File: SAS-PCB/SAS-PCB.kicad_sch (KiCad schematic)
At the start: 23 parts, among them J1_Batt1 691137710002, J2-LCD1 Conn_01x04_Socket, J3-LCD2 Conn_01x04_Socket, J4-BMP280 Conn_01x06_Pin, J5-GPS1 Conn_01x04_Socket, J6-cable-plat1 Conn_02x20_Odd_Even, J7-RFD900x1 691137710002, J8-Fan1 Conn_01x04_Socket, J9-Fan2 Conn_01x04_Socket

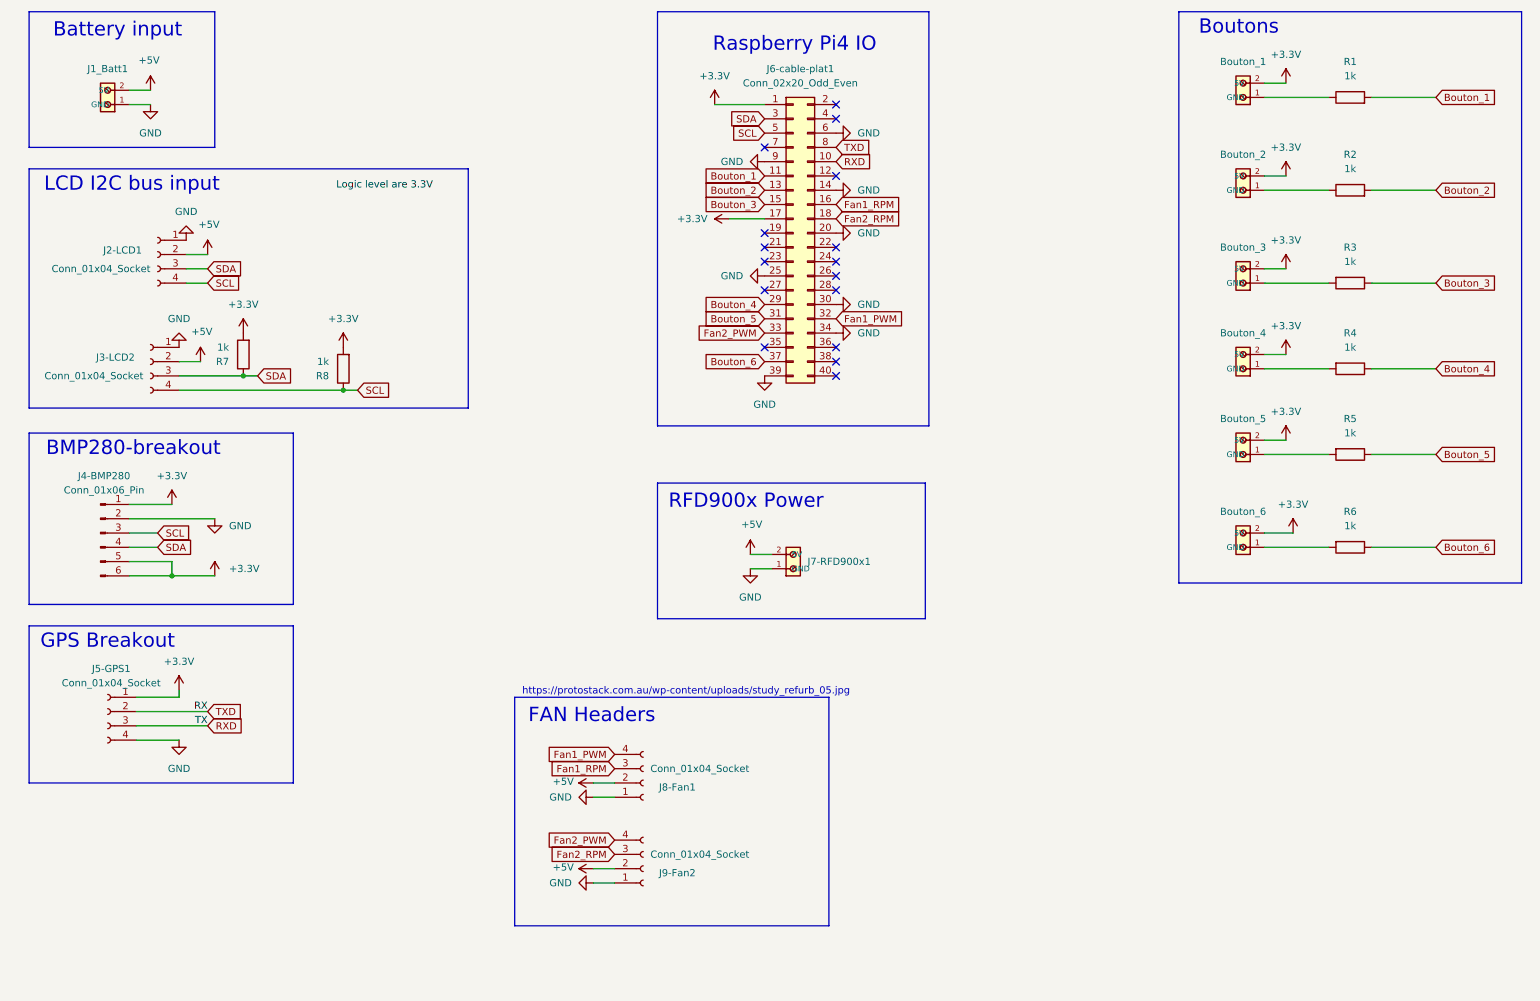
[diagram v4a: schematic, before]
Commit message: U2
trial 2
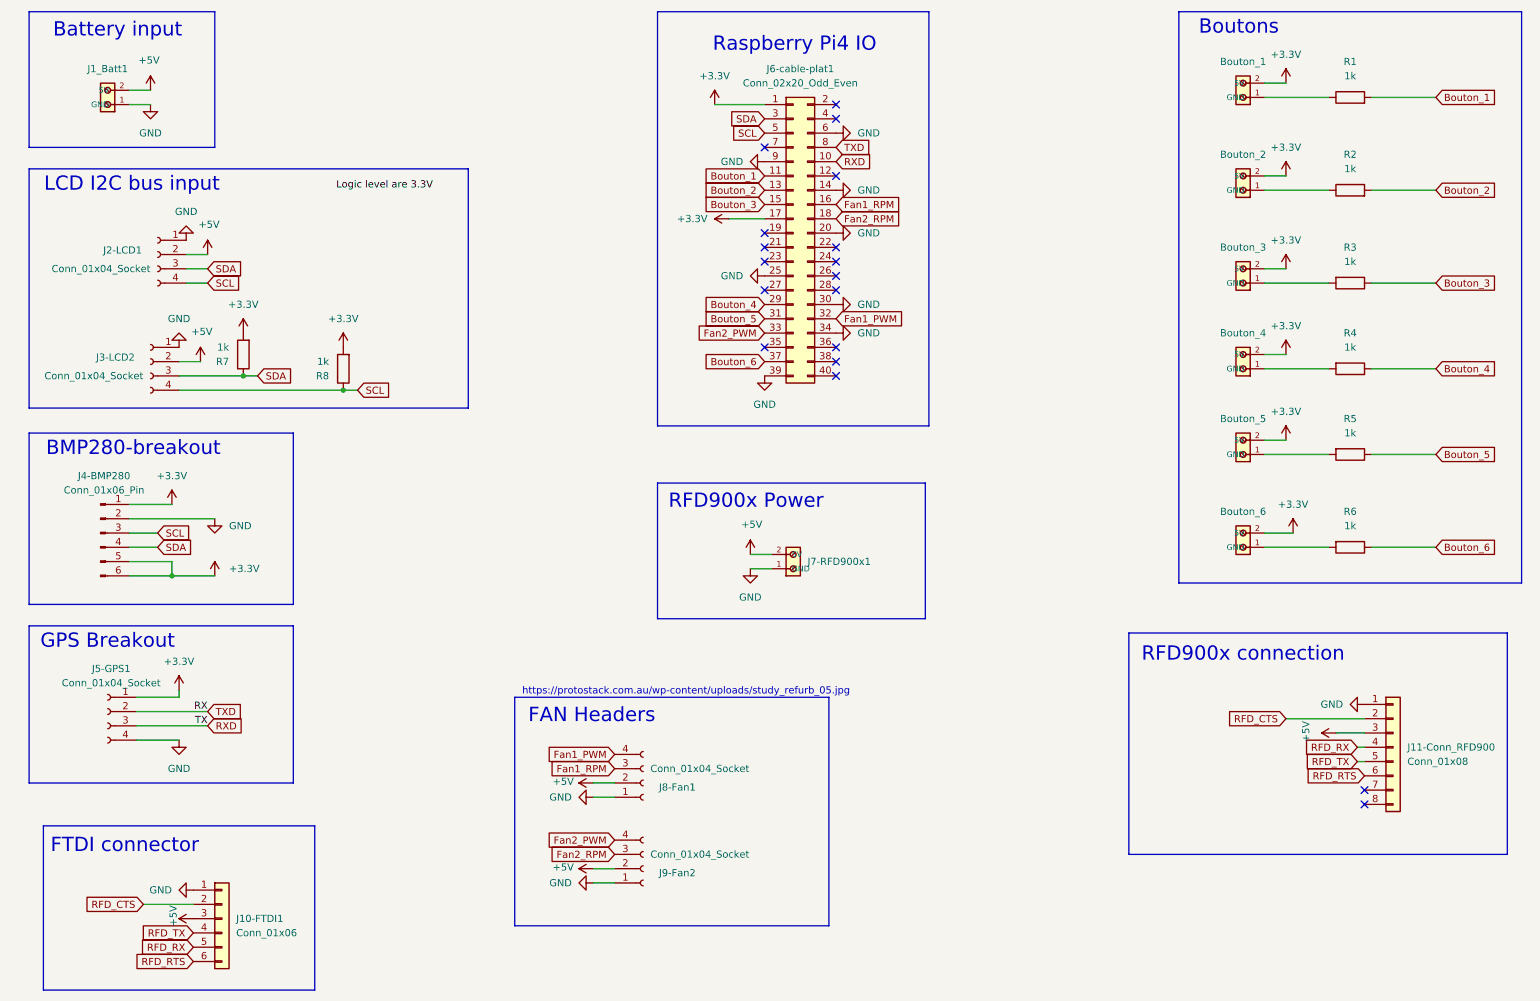
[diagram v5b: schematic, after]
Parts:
- added J10-FTDI1: Conn_01x06, SAS-Librarie-Empreinte:Conn_6_pos, symbol Connector_Generic:Conn_01x06
- added J11-Conn_RFD900: Conn_01x08, SAS-Librarie-Empreinte:Conn_8_pos, symbol Connector_Generic:Conn_01x08
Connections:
- net +5V: now also J10-FTDI1.3 (Pin_3), J11-Conn_RFD900.3 (Pin_3)
- net GND: now also J10-FTDI1.1 (Pin_1), J11-Conn_RFD900.1 (Pin_1)
- new net RFD_CTS: J10-FTDI1.2 (Pin_2), J11-Conn_RFD900.2 (Pin_2)
- new net RFD_RTS: J10-FTDI1.6 (Pin_6), J11-Conn_RFD900.6 (Pin_6)
- new net RFD_RX: J10-FTDI1.5 (Pin_5), J11-Conn_RFD900.4 (Pin_4)
- new net RFD_TX: J10-FTDI1.4 (Pin_4), J11-Conn_RFD900.5 (Pin_5)
- no-connect marks 16 -> 18
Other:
- note added: "FTDI connector"
- note added: "RFD900x connection"

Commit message: Version_a_amiliorer
pas tant fonctionnel
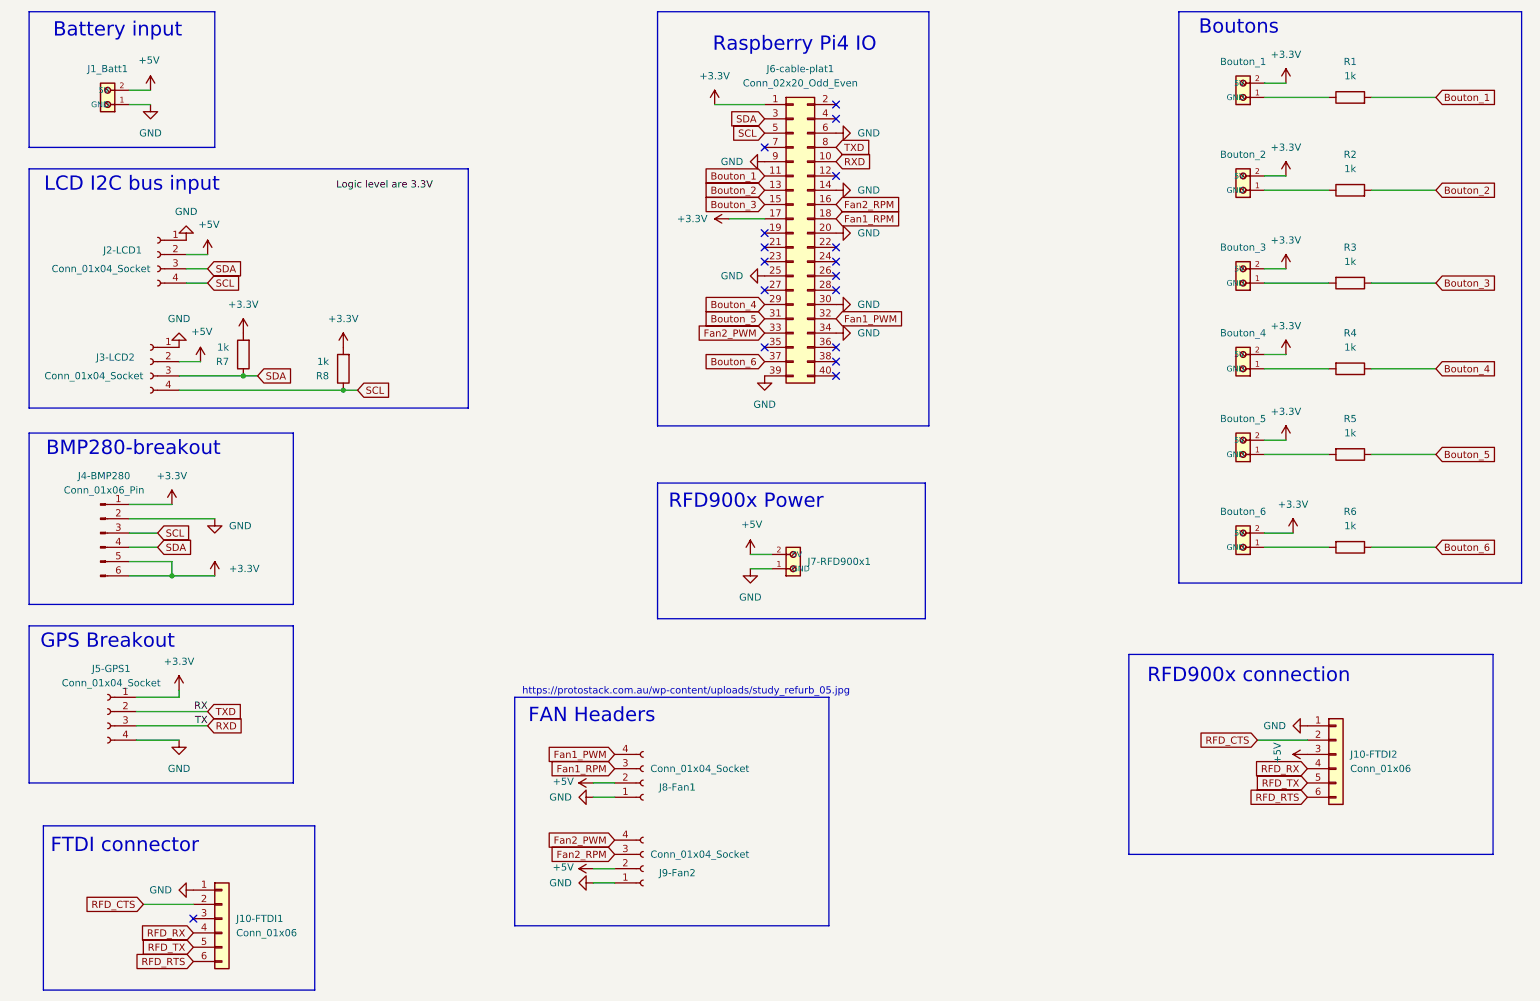
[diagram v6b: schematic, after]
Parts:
- removed J11-Conn_RFD900: Conn_01x08, SAS-Librarie-Empreinte:Conn_8_pos, symbol Connector_Generic:Conn_01x08
- added J10-FTDI2: Conn_01x06, SAS-Librarie-Empreinte:Conn_6_pos, symbol Connector_Generic:Conn_01x06
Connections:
- net +5V: now also J10-FTDI2.3 (Pin_3); no longer J10-FTDI1.3 (Pin_3)
- net Fan1_RPM: now also J6-cable-plat1.18 (Pin_18); no longer J6-cable-plat1.16 (Pin_16)
- net Fan2_RPM: now also J6-cable-plat1.16 (Pin_16); no longer J6-cable-plat1.18 (Pin_18)
- net GND: now also J10-FTDI2.1 (Pin_1)
- net RFD_CTS: now also J10-FTDI2.2 (Pin_2)
- net RFD_RTS: now also J10-FTDI2.6 (Pin_6)
- net RFD_RX: now also J10-FTDI1.4 (Pin_4), J10-FTDI2.4 (Pin_4); no longer J10-FTDI1.5 (Pin_5)
- net RFD_TX: now also J10-FTDI1.5 (Pin_5), J10-FTDI2.5 (Pin_5); no longer J10-FTDI1.4 (Pin_4)
- no-connect marks 18 -> 17
